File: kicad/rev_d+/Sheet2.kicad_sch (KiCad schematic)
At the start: 172 parts, among them J10 vg_old, J6 JUMPER, J8 JUMPER, J9 JUMPER, Q2 QUARTZ, Q3 QUARTZ32768, X11 KEYB-MOUSE, X12 IDC20, X13 USB_C, X15 PLB2-2, X19 AVR pgm conn, X21 Turbosound conn, X22 PS2 extra input, X23 SEGA pads, X3 IDC26LPT, X4 IDC10M, X5 IDC10M, X6 RS232_9

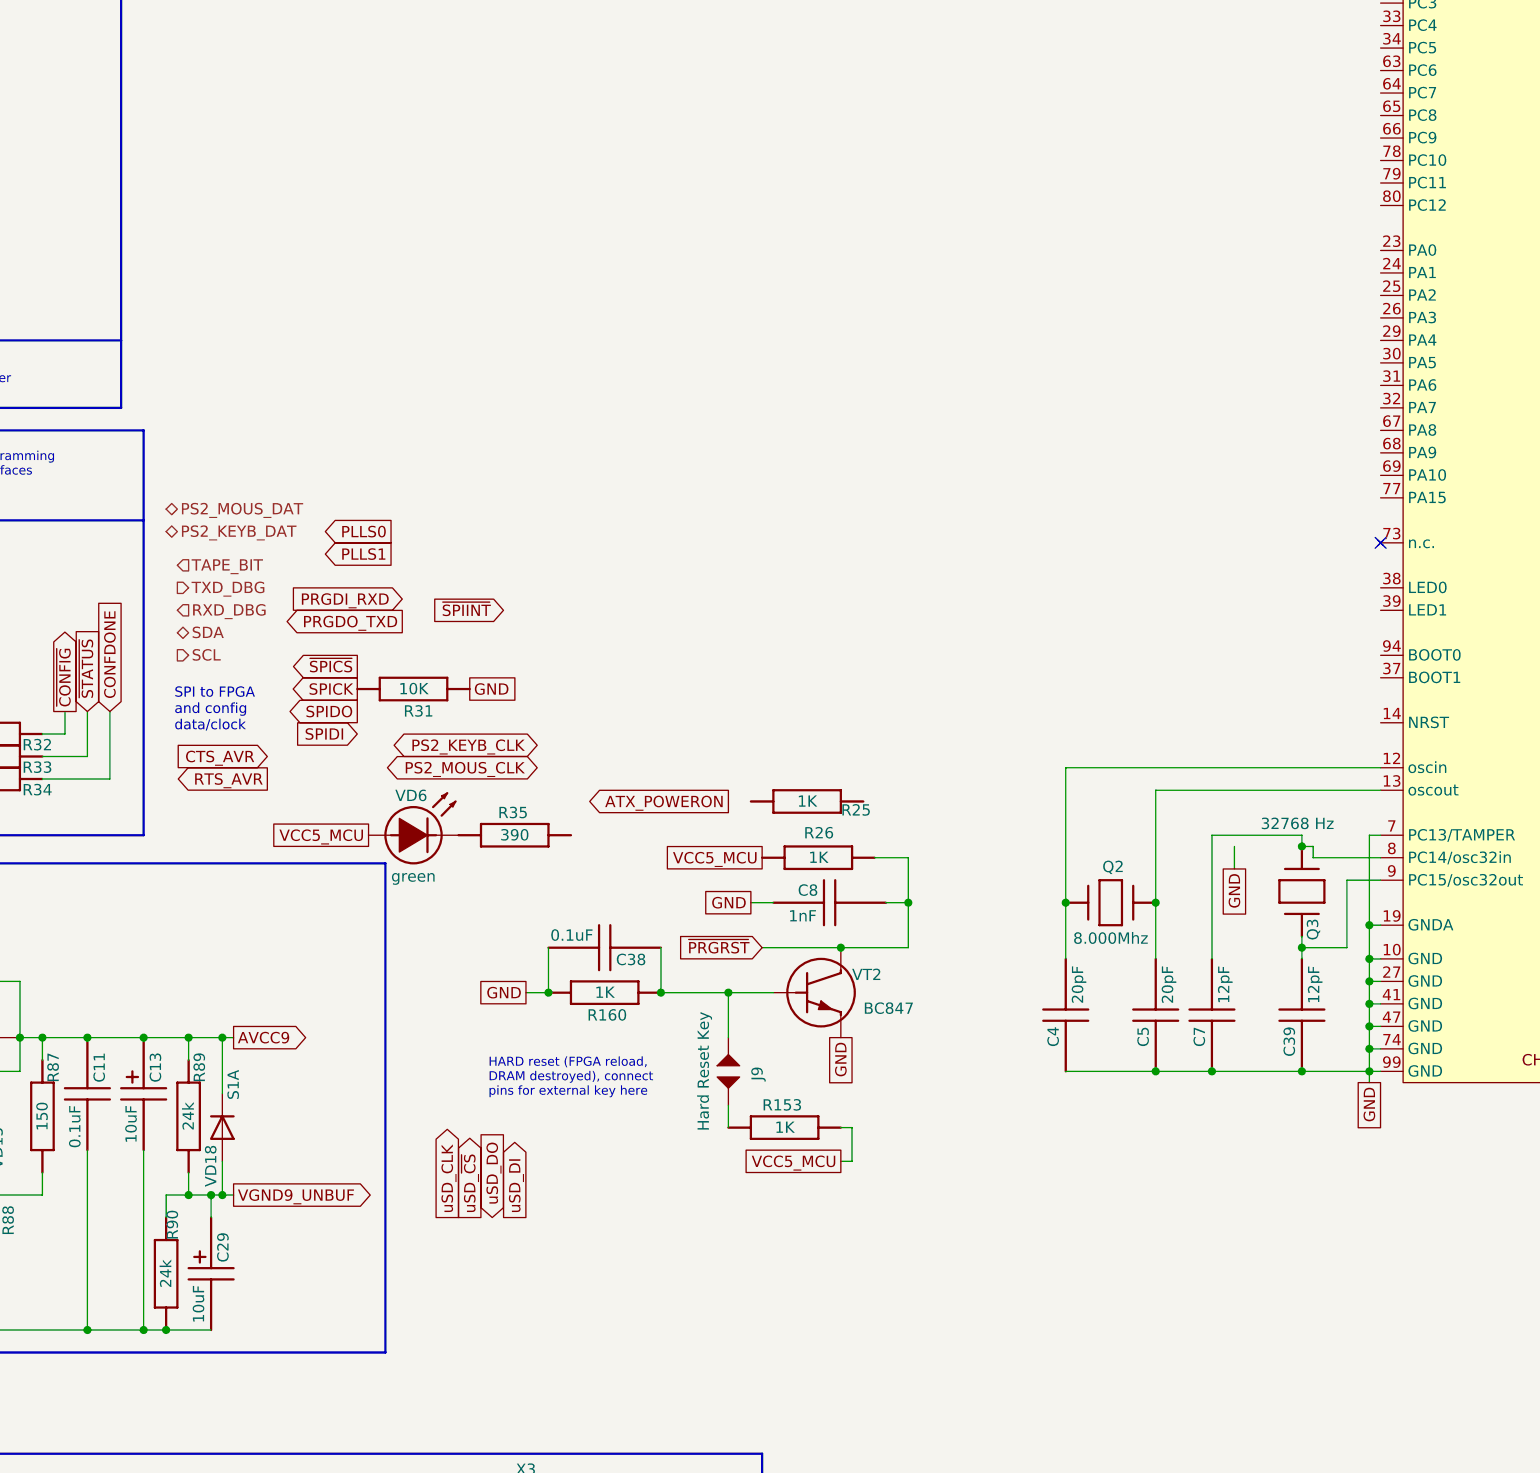
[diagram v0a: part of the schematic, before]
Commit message: pentevo: rev D+:
git-svn-id: svn://localhost/local-pentevo@1291 c6c76956-fad2-4150-a3a9-ea0a427205ba
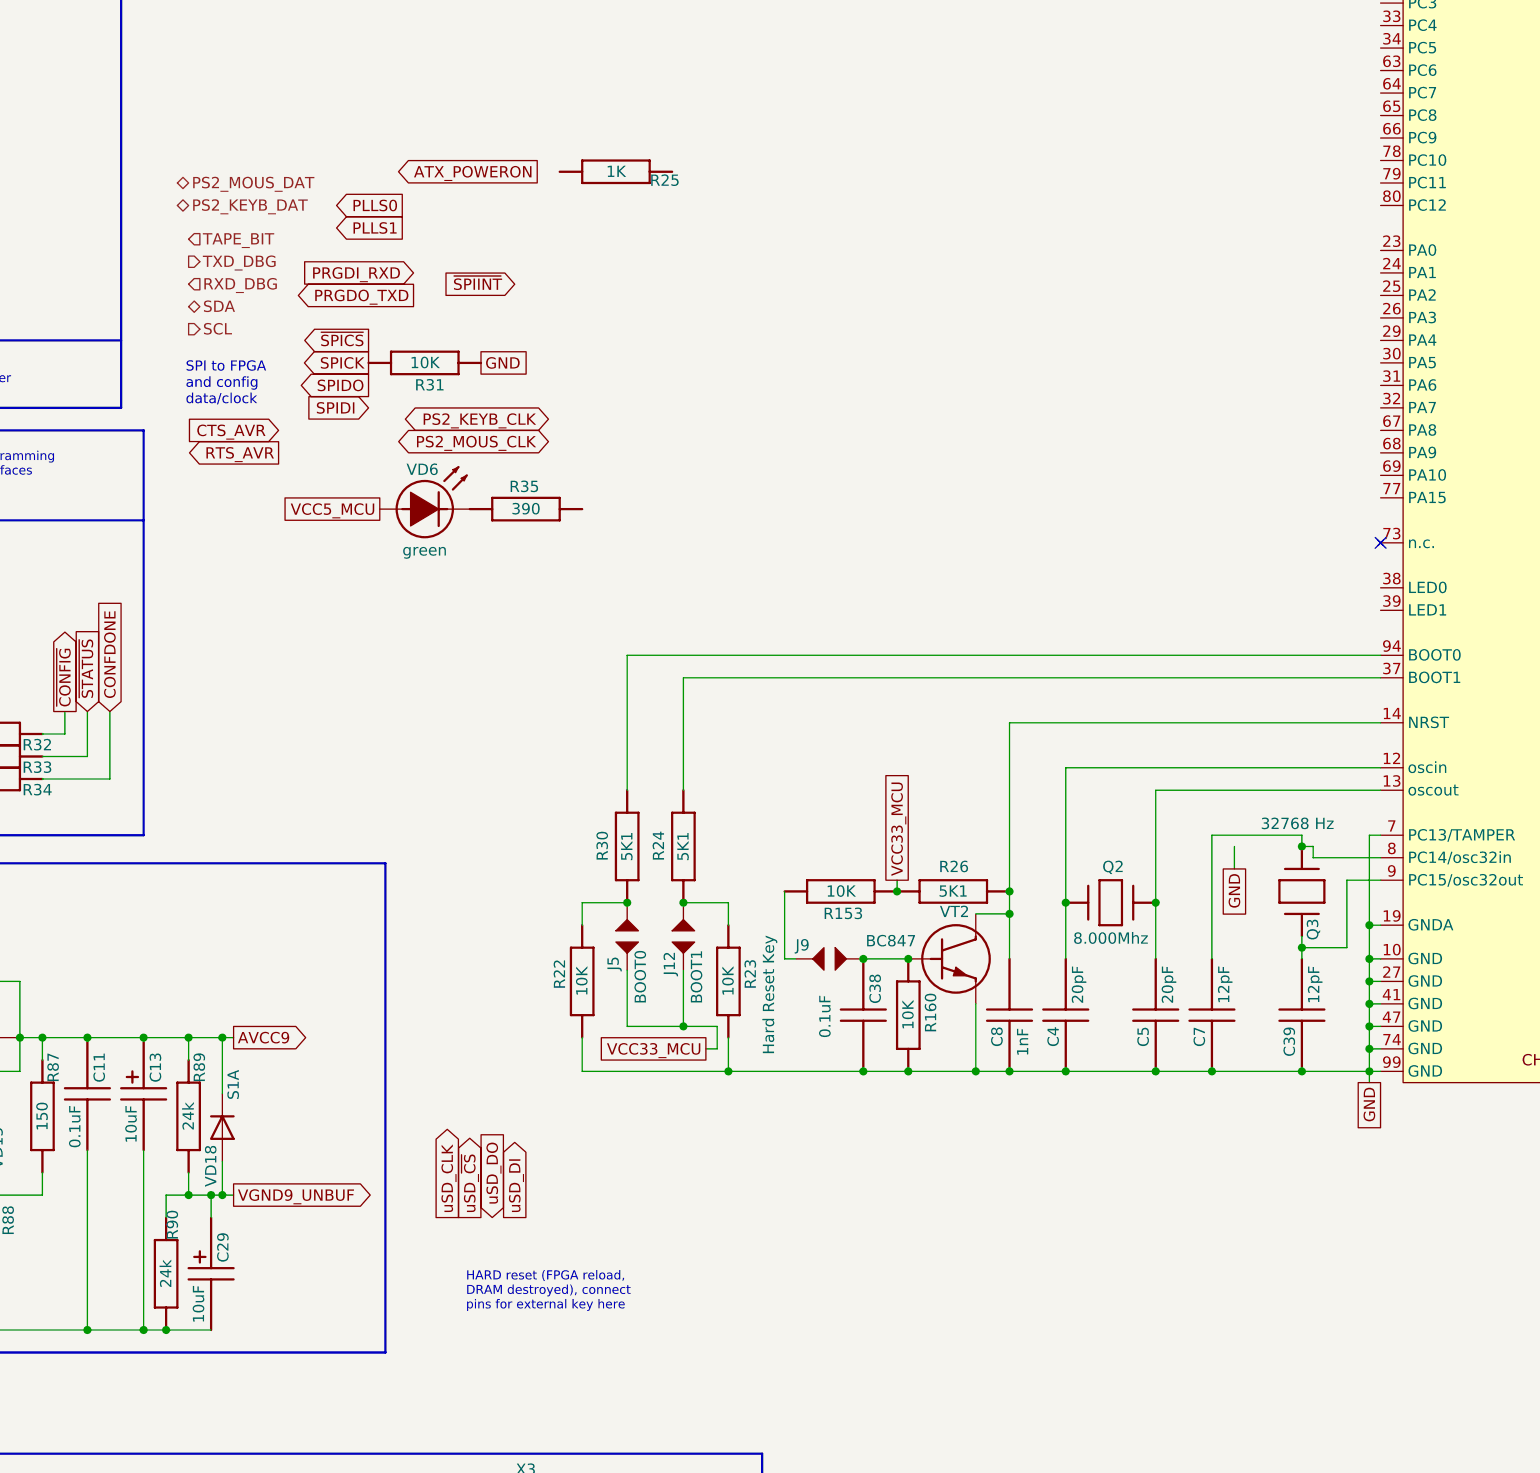
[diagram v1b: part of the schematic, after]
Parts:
- added J12, J5: JUMPER, JUMPER, symbol eva-altium-import:Sheet2_3_JUMPER
- added R22, R23: 10K, R-CHIP, symbol eva-altium-import:Sheet2_0_mirrored_RESCHIP
- added R24, R30: 5K1, R-CHIP, symbol eva-altium-import:Sheet2_0_RESCHIP
- R153, R160: value 1K -> 10K
- R26: value 1K -> 5K1
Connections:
- net GND: now also R22.2 (i/o1), R23.2 (i/o1)
- net VCC33_MCU: now also R153.1 (i/o), R26.2 (i/o1), J12.1 (2), J5.1 (2)
- net VCC5_MCU: no longer R153.2 (i/o1), R26.2 (i/o1)
- net ~{PRGRST}: no longer C8.2, R26.1 (i/o), VT2.3 (collector)
- net at J9.1 (2): now also R153.2 (i/o1); no longer R153.1 (i/o)
- net at D4.14 (NRST): now also C8.2, R26.1 (i/o), VT2.3 (collector)
- net at D4.37 (BOOT1): now also R24.1 (i/o)
- net at D4.94 (BOOT0): now also R30.1 (i/o)
- new net: J5.0 (1), R22.1 (i/o), R30.2 (i/o1)
- new net: J12.0 (1), R23.1 (i/o), R24.2 (i/o1)
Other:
- moved on the sheet: C38, C8, J9, R153, R160, R25, R26, R31, R35, VD6, VT2
